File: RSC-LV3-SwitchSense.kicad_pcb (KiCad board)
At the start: 2 copper layers, 140 x 85 mm, 171 parts, among them J1 FTSH-105-01-L-DV-K-A, J10 Molex 43045-0400, J11 Molex 43045-0400, J12 Molex 43045-0400, J13 Molex 43045-0400, J14 Molex 43045-0400, J15 Molex 43045-0400, J16 Molex 43650-0200, J2 USB_C_Receptacle_USB2.0_16P, J3 Molex 43650-0500, J4 Molex 43650-0500, J5 Molex 43650-0200, J6 Molex 43045-0400, J7 Molex 43045-0400, J8 Molex 43045-0400, J9 Molex 43045-0400, Q1 AO3400A, Q10 AO3400A, Q2 AO3400A, Q3 AO3400A, Q4 AO3400A, Q5 AO3400A, Q6 AO3400A, Q7 AO3400A, Q8 AO3400A, Q9 AO3400A, U1 STM32G0B1CBTx, U2 TPS54302, U3 TLV74033PDBVR, U4 TJA1051T-3, U5 TJA1051T-3, Y1 Crystal_GND24, Y2 32.768 kHz 6pF

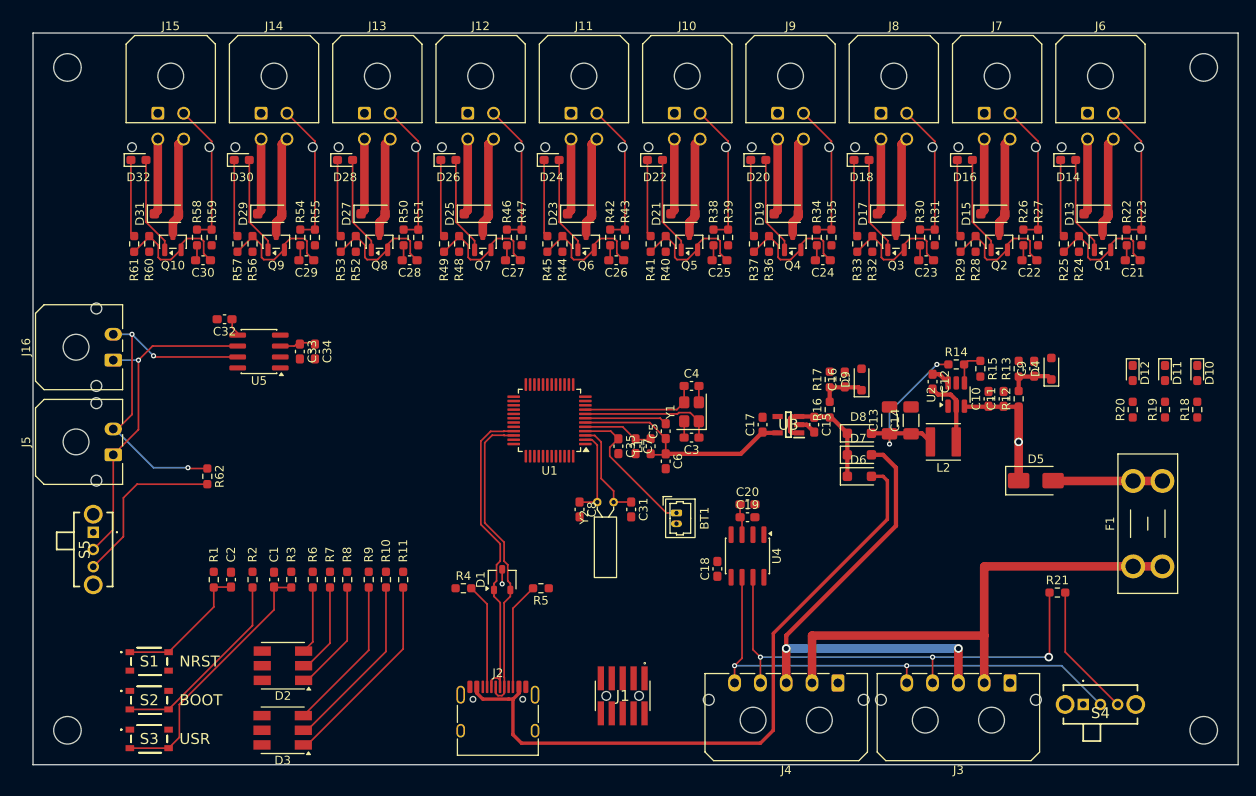
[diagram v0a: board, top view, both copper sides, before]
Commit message: initial complete route
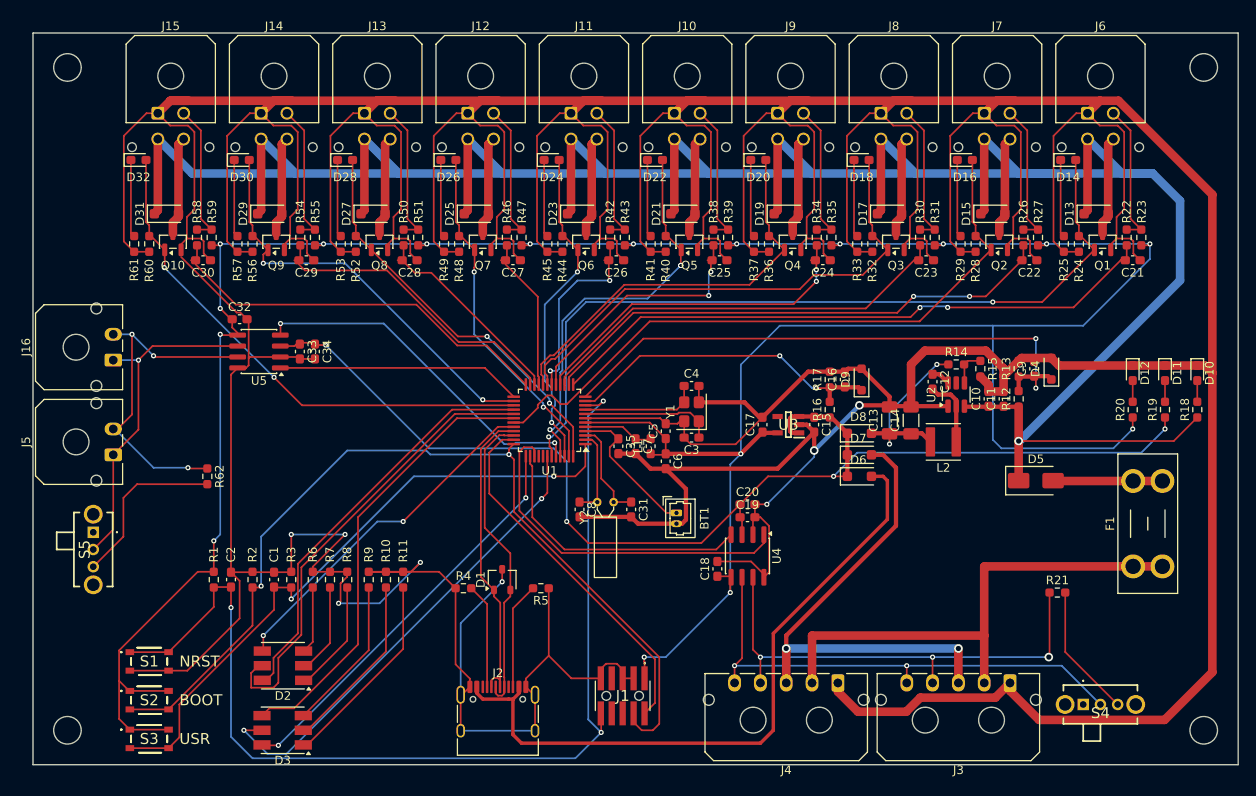
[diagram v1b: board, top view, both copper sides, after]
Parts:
- moved C32 1.75 mm to (94.0, 83.2), turned to 0 degrees
- turned R24 to -90 degrees
- turned R28 to -90 degrees
- turned R32 to -90 degrees
- turned R36 to -90 degrees
- turned R40 to -90 degrees
- turned R44 to -90 degrees
- turned R48 to -90 degrees
- turned R52 to -90 degrees
- turned R56 to -90 degrees
- turned R60 to -90 degrees
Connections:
- J2 pad SH: (no net) -> GND
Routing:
- net GND: track 167.5 -> 1127.5 mm, vias 1 -> 8
- net +3.3V: track 29.8 -> 355.7 mm, vias 0 -> 17
- net +12V: track 103.5 -> 341.3 mm
- net +5V: track 23.0 -> 143.9 mm, vias 0 -> 4
- net NRST: track 16.2 -> 123.2 mm, vias 0 -> 3
- net BOOT0: track 22.7 -> 107.3 mm, vias 0 -> 2
- net OUT_1: track 11.2 -> 93.0 mm, vias 0 -> 2
- net IN_1: track 1.80 -> 72.0 mm, vias 0 -> 2
- net OUT_2: track 11.2 -> 76.2 mm
- net V_SENSE_12: track 5.66 -> 68.0 mm, vias 0 -> 2
- net IN_2: track 1.80 -> 61.5 mm, vias 0 -> 2
- net STAT1_G: track 0.00 -> 55.3 mm, vias 0 -> 2
- net STAT0_G: track 0.00 -> 53.3 mm
- net STAT1_B: track 0.00 -> 52.2 mm
- net OUT_10: track 11.2 -> 60.7 mm, vias 0 -> 2
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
